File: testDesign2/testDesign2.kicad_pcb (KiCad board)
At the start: 2 copper layers, 25 x 26.3 mm, 31 parts, among them SW1 SW_Push, U1 CC2640R2FRSM, Y1 32.768kHz, Y2 24MHz

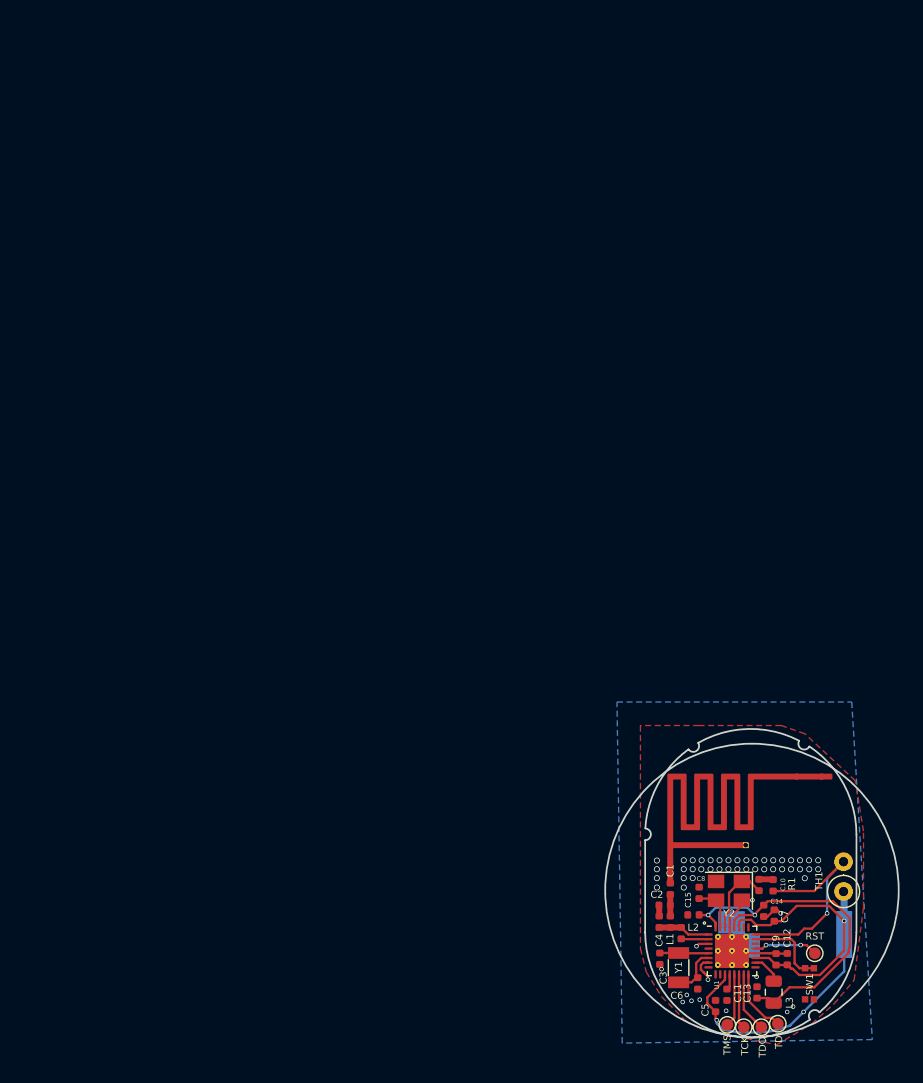
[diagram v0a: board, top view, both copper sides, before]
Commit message: Think PCB design is finished. Need to do last checkthrough.
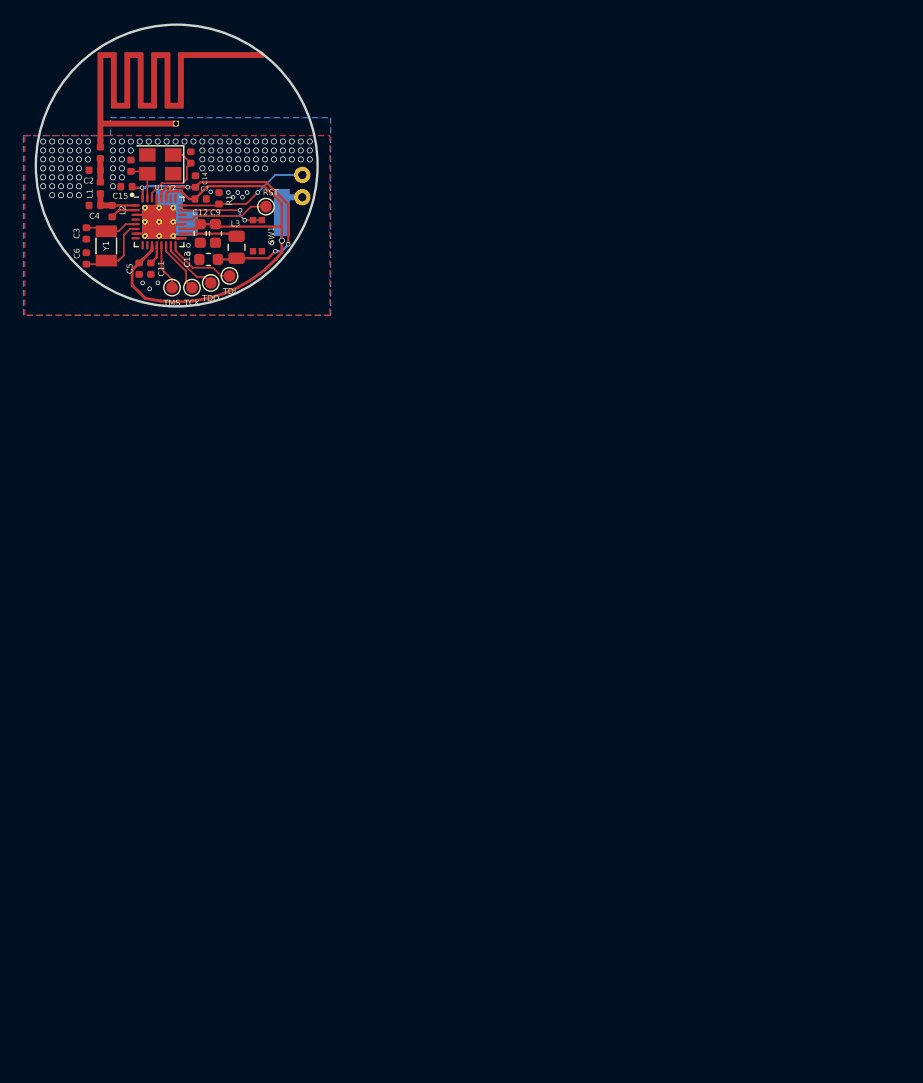
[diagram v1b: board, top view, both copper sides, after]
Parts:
- C12, C13, C9: footprint Capacitor_SMD:C_0402_1005Metric -> Capacitor_SMD:C_0603_1608Metric
- TH1: footprint Resistor_THT:R_Axial_DIN0207_L6.3mm_D2.5mm_P2.54mm_Vertical -> Resistor_THT:R_Axial_DIN0204_L3.6mm_D1.6mm_P1.90mm_Vertical; moved to B.Cu
- moved C6 80.8 mm to (49.8, 57.2), turned to 90 degrees
- moved C5 79.7 mm to (54.3, 58.1), turned to 270 degrees
- moved C12 79.5 mm to (59.5, 55.1), turned to 270 degrees
- moved C1 79.3 mm to (51.0, 48.2)
- moved C2 79.2 mm to (50.5, 49.7)
- moved SW1 79.2 mm to (64.4, 55.3)
- moved L1 79.1 mm to (51.0, 51.2)
- moved TDI 79.0 mm to (62.0, 58.7), turned to 180 degrees
- moved U1 79.0 mm to (56.0, 54.1)
- moved C11 79.0 mm to (55.3, 58.1)
- moved RST 78.9 mm to (65.1, 52.8), turned to 180 degrees
- moved TDO 78.9 mm to (60.4, 59.3), turned to 180 degrees
- moved C3 78.8 mm to (49.8, 55.1)
- moved C14 78.8 mm to (59.1, 50.7), turned to 90 degrees
- moved C10 78.6 mm to (58.7, 48.6)
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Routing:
- net ADC0: track 19.0 -> 11.3 mm
- net GND: track 16.5 -> 11.4 mm, vias 53 -> 116
- net VDDR: track 31.5 -> 28.2 mm, vias 2 -> 4
- net Net-(C6-Pad1): track 4.04 -> 6.46 mm
- net Net-(TP11-Pad1): track 5.46 -> 7.56 mm, vias 2 -> 0
- net DCDC_SW: track 2.55 -> 4.30 mm
- net Net-(AE1-Pad1): track 1.78 -> 0.73 mm
- net Net-(C3-Pad1): track 3.59 -> 4.57 mm
- net Net-(TP4-Pad1): track 4.55 -> 3.97 mm
- net VDDS: track 47.5 -> 47.1 mm, vias 3 -> 1
- net Button: track 7.04 -> 7.37 mm, vias 0 -> 2
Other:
- board size 25 x 26.3 mm -> 24 x 24 mm
- net class Default: clearance 0.2 -> 0.1524; trace_width 0.25 -> 0.1524; via_dia 0.8 -> 0.381; via_drill 0.4 -> 0.254
- rule pad_to_mask_clearance: 0.051 -> 0
- rule trace_clearance: 0.2 -> 0.1524
